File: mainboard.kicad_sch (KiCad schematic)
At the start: 29 parts, among them J1 terminal_led-strip, J2 header_rotary-encoder, J4 header_pi, J5 power_input, J6 AudioJack2, Q1 IRF9540N, SW1 power_switch, U1 OPA2277, U2 MSGEQ7, U4 logic-level-converter, U5 logic-level-converter

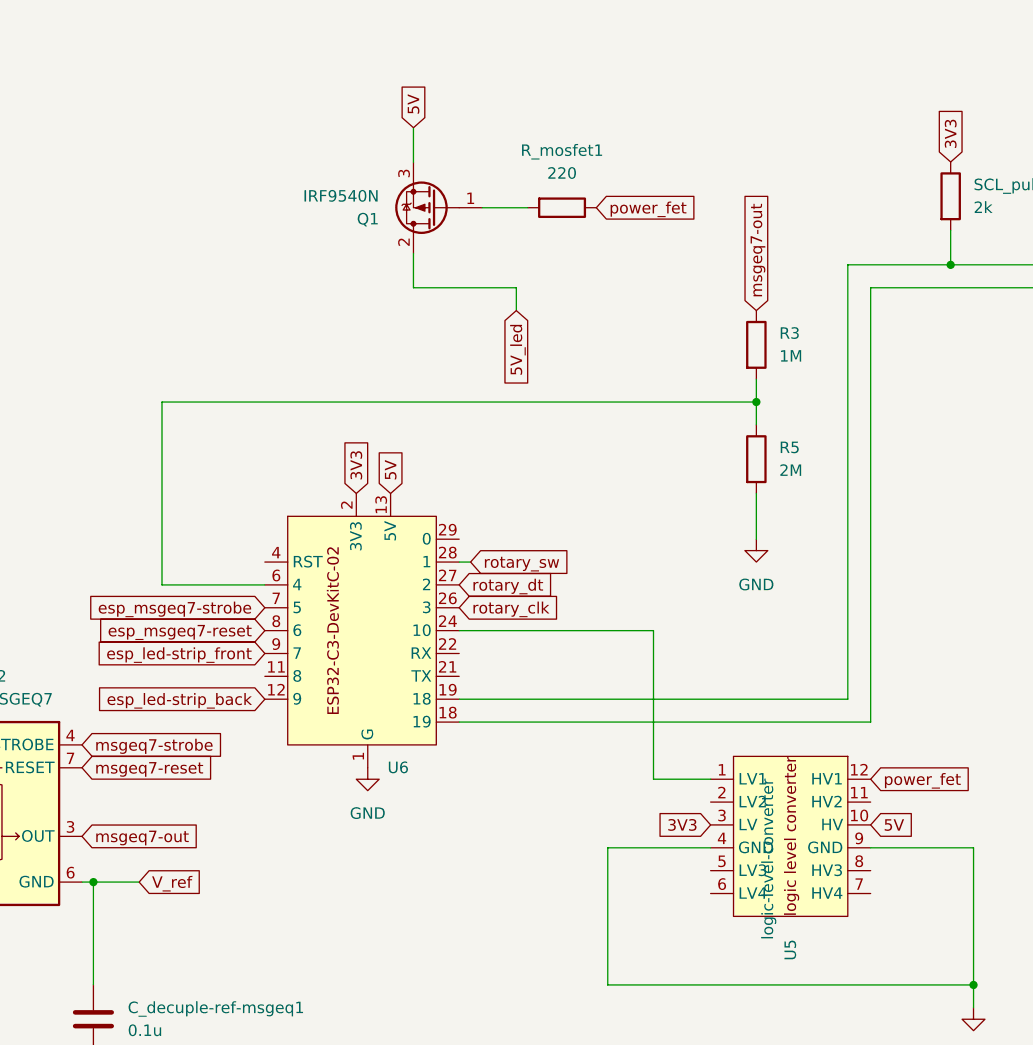
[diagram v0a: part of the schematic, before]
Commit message: route tracks and add mounting holes
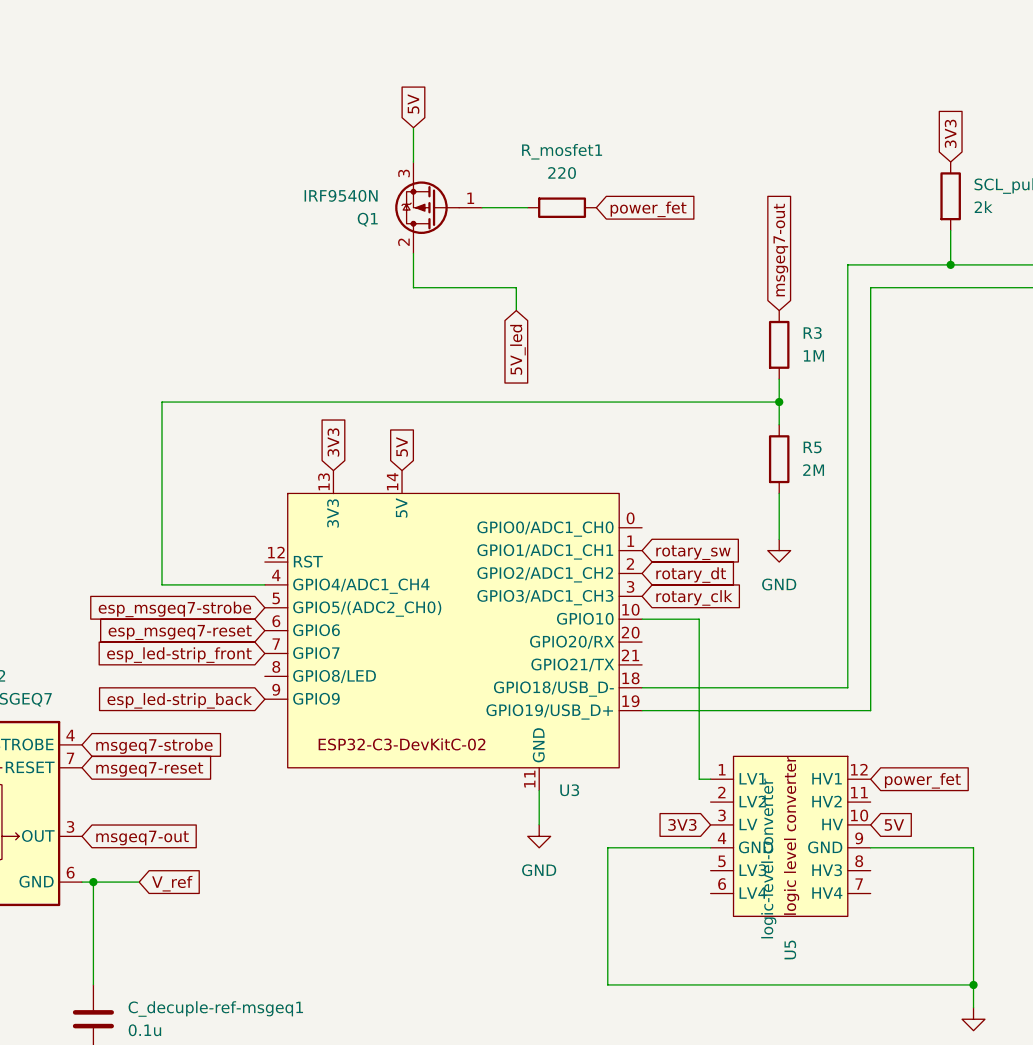
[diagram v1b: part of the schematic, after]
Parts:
- removed U6: ~, my_lib:esp32_c3_dev-kit-c_02, symbol my_lib:esp32_c3_dev-kit-c_02
- added U3: ~, my_lib:esp32_c3_dev-kit-c_02, symbol my_lib:esp32_c3_dev-kit-c_02
- C1, C_clock-msgeq1, C_decouple-supply1, C_decuple-ref-msgeq1: footprint Capacitor_SMD:C_0603_1608Metric_Pad1.08x0.95mm_HandSolder -> Capacitor_SMD:C_0805_2012Metric_Pad1.18x1.45mm_HandSolder
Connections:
- net 3V3: now also U3.13 (3V3)
- net 5V: now also U3.14 (5V)
- net GND: now also U3.11 (GND)
- net esp_led-strip_back: now also U3.9 (GPIO9)
- net esp_led-strip_front: now also U3.7 (GPIO7)
- net esp_msgeq7-reset: now also U3.6 (GPIO6)
- net esp_msgeq7-strobe: now also U3.5 (GPIO5/(ADC2_CH0))
- net rotary_clk: now also U3.3 (GPIO3/ADC1_CH3)
- net rotary_dt: now also U3.2 (GPIO2/ADC1_CH2)
- net rotary_sw: now also U3.1 (GPIO1/ADC1_CH1)
- net at R3.2, R5.1: now also U3.4 (GPIO4/ADC1_CH4)
- net at J4.3 (Pin_3), SDA_pullup1.2: now also U3.19 (GPIO19/USB_D+)
- net at J4.2 (Pin_2), SCL_pullup1.2: now also U3.18 (GPIO18/USB_D-)
- net at U5.1 (LV1): now also U3.10 (GPIO10)
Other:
- moved on the sheet: R3, R5
